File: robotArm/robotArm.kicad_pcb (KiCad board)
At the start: 4 copper layers, 127 x 69.9 mm, 46 parts, among them J1 Barrel_Jack, J2 Conn_01x16_Pin, J3 Conn_01x04, J4 Conn_01x04, J5 Conn_01x04, J6 Conn_01x04, U2 TMC2209_SILENTSTEPSTICK, U4 TMC2209_SILENTSTEPSTICK, U5 TMC2209_SILENTSTEPSTICK, U6 74HC165

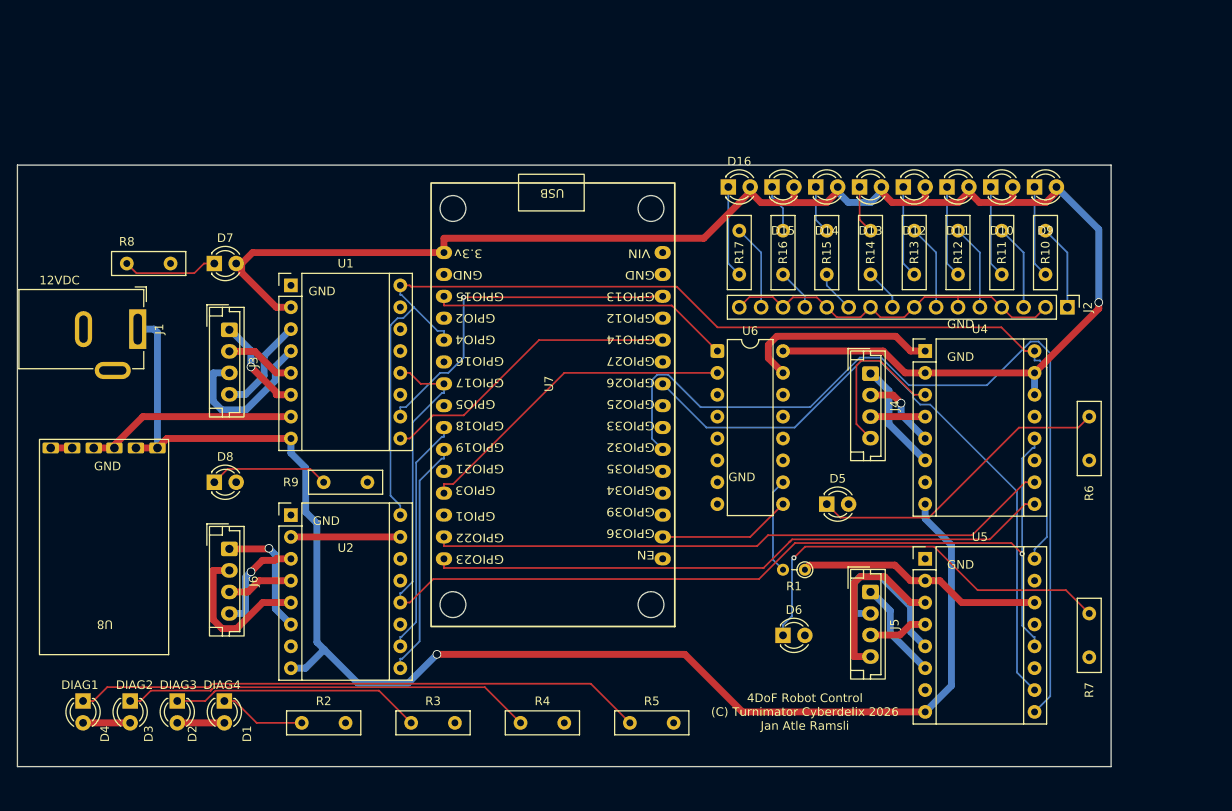
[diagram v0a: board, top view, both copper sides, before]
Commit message: Attempt 2.1
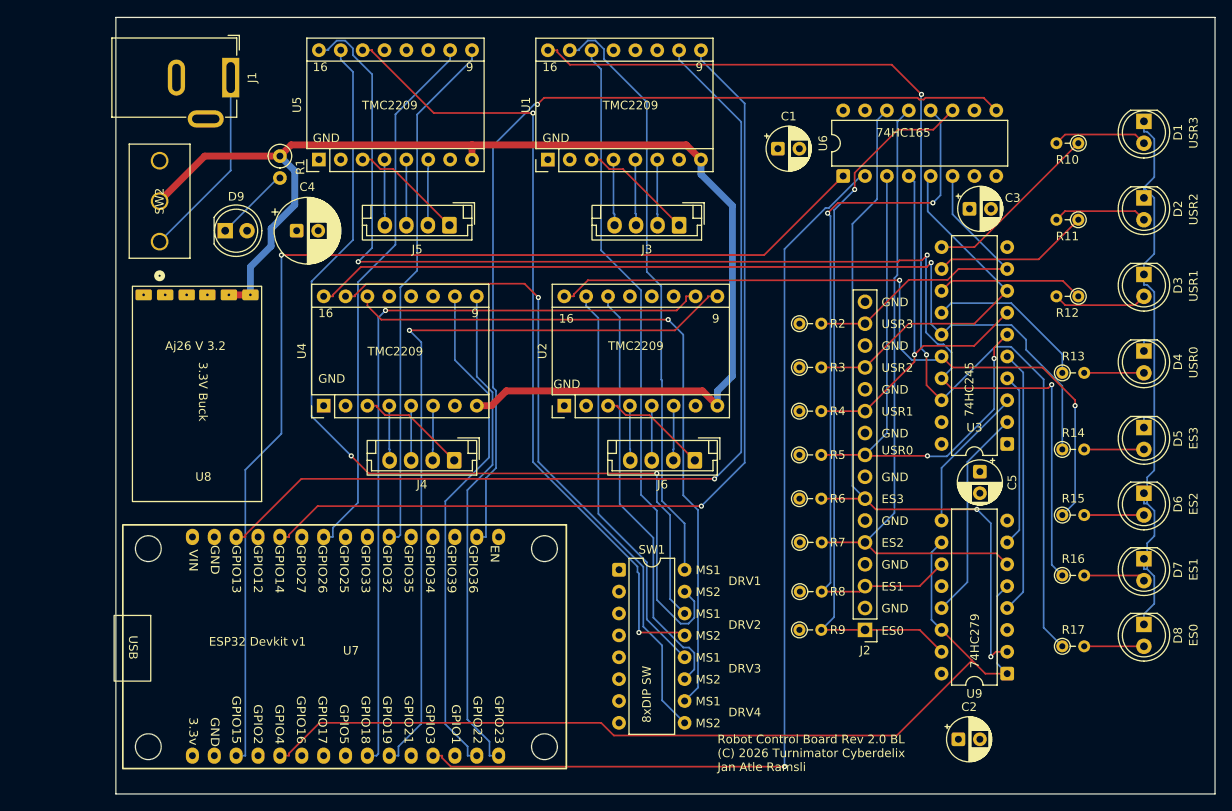
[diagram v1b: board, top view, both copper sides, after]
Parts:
- removed D10: ST1, LED_THT:LED_D3.0mm_FlatTop
- removed D11: ST2, LED_THT:LED_D3.0mm_FlatTop
- removed D12: ST3, LED_THT:LED_D3.0mm_FlatTop
- removed D13: USR0, LED_THT:LED_D3.0mm_FlatTop
- removed D14: USR1, LED_THT:LED_D3.0mm_FlatTop
- removed D15: USR2, LED_THT:LED_D3.0mm_FlatTop
- removed D16: USR3, LED_THT:LED_D3.0mm_FlatTop
- added C1: 47μ, Capacitor_THT:CP_Radial_D5.0mm_P2.50mm, F.Cu at (113.7, 60.3)
- added C2: 47μ, Capacitor_THT:CP_Radial_D5.0mm_P2.50mm, F.Cu at (134.7, 128.9)
- added C3: 47μ, Capacitor_THT:CP_Radial_D5.0mm_P2.50mm, F.Cu at (136.0, 67.3)
- added C4: 100μ, Capacitor_THT:CP_Radial_D7.5mm_P2.50mm, F.Cu at (57.8, 69.8)
- added C5: 47μ, Capacitor_THT:CP_Radial_D5.0mm_P2.50mm, F.Cu at (137.2, 97.8)
- added SW1: SW_DIP_x08, Package_DIP:DIP-16_W7.62mm, F.Cu at (95.3, 109.2)
- added SW2: SW_SPDT, Library:SS-12D10G5_XKB, F.Cu at (41.9, 71.1)
- added U3: 74HC245, Package_DIP:DIP-20_W7.62mm, F.Cu at (140.3, 94.6)
- added U9: 74LS279, Package_DIP:DIP-16_W7.62mm, F.Cu at (140.3, 121.3)
- D1: value DIAG1 -> USR3; footprint LED_THT:LED_D3.0mm_FlatTop -> LED_THT:LED_D5.0mm
- D2: value DIAG2 -> USR2; footprint LED_THT:LED_D3.0mm_FlatTop -> LED_THT:LED_D5.0mm
- D3: value DIAG3 -> USR1; footprint LED_THT:LED_D3.0mm_FlatTop -> LED_THT:LED_D5.0mm
- D4: value DIAG4 -> USR0; footprint LED_THT:LED_D3.0mm_FlatTop -> LED_THT:LED_D5.0mm
- D5: value IX1 -> ES3; footprint LED_THT:LED_D3.0mm_FlatTop -> LED_THT:LED_D5.0mm
- D6: value IX2 -> ES2; footprint LED_THT:LED_D3.0mm_FlatTop -> LED_THT:LED_D5.0mm
- D7: value IX3 -> ES1; footprint LED_THT:LED_D3.0mm_FlatTop -> LED_THT:LED_D5.0mm
- D8: value IX4 -> ES0; footprint LED_THT:LED_D3.0mm_FlatTop -> LED_THT:LED_D5.0mm
- D9: value ST0 -> LED; footprint LED_THT:LED_D3.0mm_FlatTop -> LED_THT:LED_D5.0mm_Clear
- J2: value Conn_01x16_Pin -> ENDSTOP INPUTS
- J3: value Conn_01x04 -> STEPPER1
- J4: value Conn_01x04 -> STEPPER4
- J5: value Conn_01x04 -> STEPPER2
- J6: value Conn_01x04 -> STEPPER3
- R1: value R -> 470 Ω; footprint Resistor_THT:R_Axial_DIN0204_L3.6mm_D1.6mm_P2.54mm_Vertical -> Resistor_THT:R_Axial_DIN0207_L6.3mm_D2.5mm_P2.54mm_Vertical
- R10, R11, R12, R13, R14, R15, R16, R17: value 330 -> 330Ω; footprint Resistor_THT:R_Box_L8.4mm_W2.5mm_P5.08mm -> Resistor_THT:R_Axial_DIN0204_L3.6mm_D1.6mm_P2.54mm_Vertical
- R2, R3, R4, R5, R6, R7, R8, R9: value 330 -> 10kΩ; footprint Resistor_THT:R_Box_L8.4mm_W2.5mm_P5.08mm -> Resistor_THT:R_Axial_DIN0204_L3.6mm_D1.6mm_P2.54mm_Vertical
- U4: value TMC2209_SILENTSTEPSTICK -> TMC2209_MODULE
- U5: value TMC2209_SILENTSTEPSTICK -> TMC2209 Module
- moved D4 129.7 mm to (156.2, 83.8)
- moved D3 127.7 mm to (156.2, 74.9)
- moved D2 126.5 mm to (156.2, 66.0)
- moved D1 126.2 mm to (156.2, 57.1)
- moved D7 113.3 mm to (156.2, 108.0), turned to -90 degrees
- moved D8 109.2 mm to (156.2, 115.6), turned to -90 degrees
- moved D9 94.1 mm to (49.5, 69.8)
- moved R8 86.9 mm to (116.3, 111.8)
- moved U5 84.3 mm to (60.4, 61.6), turned to 90 degrees
- moved R1 77.6 mm to (55.9, 61.2), turned to -90 degrees
- moved R2 74.1 mm to (116.2, 80.6)
- moved U4 70.1 mm to (61.0, 90.2), turned to 90 degrees
- moved J5 64.8 mm to (75.6, 69.2), turned to 180 degrees
- moved R3 61.1 mm to (116.2, 85.7)
- moved R9 57.8 mm to (116.2, 116.2)
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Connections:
- D1 pad 2: +3.3V -> Net-(D1-A)
- D2 pad 1: Net-(D2-K) -> Net-(D1-K)
- D2 pad 2: +3.3V -> Net-(D2-A)
- D3 pad 1: Net-(D3-K) -> Net-(D1-K)
- D3 pad 2: +3.3V -> Net-(D3-A)
- D4 pad 1: Net-(D4-K) -> Net-(D1-K)
- D4 pad 2: +3.3V -> Net-(D4-A)
- D5 pad 1: Net-(D5-K) -> Net-(D1-K)
- D5 pad 2: +3.3V -> Net-(D5-A)
- D6 pad 1: Net-(D6-K) -> Net-(D1-K)
- D6 pad 2: +3.3V -> Net-(D6-A)
- D7 pad 1: Net-(D7-K) -> Net-(D1-K)
- D7 pad 2: +3.3V -> Net-(D7-A)
- D8 pad 1: Net-(D8-K) -> Net-(D1-K)
- D8 pad 2: +3.3V -> Net-(D8-A)
- D9 pad 2: +3.3V -> GND
- J1 pad 1: +12V -> Net-(J1-Pad1)
- J2 pad 1: ES0 -> /Endstop Section/ES0
- J2 pad 10: Net-(J2-Pin_10) -> GND
- J2 pad 11: USR1 -> /Endstop Section/USR1
- J2 pad 12: Net-(J2-Pin_10) -> GND
- J2 pad 13: USR2 -> /Endstop Section/USR2
- J2 pad 14: Net-(J2-Pin_10) -> GND
- J2 pad 15: USR3 -> /Endstop Section/USR3
- J2 pad 16: Net-(J2-Pin_10) -> GND
- J2 pad 2: Net-(J2-Pin_10) -> GND
- J2 pad 3: ES1 -> /Endstop Section/ES1
- J2 pad 4: Net-(J2-Pin_10) -> GND
- J2 pad 5: ES2 -> /Endstop Section/ES2
- J2 pad 6: Net-(J2-Pin_10) -> GND
- J2 pad 7: ES3 -> /Endstop Section/ES3
- J2 pad 8: Net-(J2-Pin_10) -> GND
- J2 pad 9: USR0 -> /Endstop Section/USR0
- J3 pad 1: /M1-2B -> /B2-DRV1
- J3 pad 2: /M1-2A -> /A2-DRV1
- J3 pad 3: /M1-1A -> /A1-DRV1
- J3 pad 4: /M1-1B -> /B1-DRV1
- J4 pad 1: /M4-1B -> /B2-DRV4
- J4 pad 2: /M4-2A -> /A2-DRV4
- J4 pad 3: /M4-1A -> /A1-DRV4
- J4 pad 4: Net-(J4-2B) -> /B1-DRV4
- J5 pad 1: /M2-2B -> /B2-DRV2
- J5 pad 2: /M2-2A -> /A2-DRV2
- J5 pad 3: /M2-1A -> /A1-DRV2
- J5 pad 4: /M2-1B -> /B1-DRV2
- J6 pad 1: /M3-2B -> /B2-DRV3
- J6 pad 2: /M3-2A -> /A2-DRV3
- J6 pad 3: /M3-1A -> /A1-DRV3
- J6 pad 4: /M3-1B -> /B1-DRV3
- R1 pad 1: +3.3V -> +12V
- R1 pad 2: Net-(U6-DS) -> Net-(D9-K)
- R10 pad 1: Net-(D9-K) -> Net-(U3-B7)
- R10 pad 2: ES0 -> Net-(D1-A)
- R11 pad 2: ES1 -> Net-(D2-A)
- R12 pad 2: ES2 -> Net-(D3-A)
- R13 pad 2: ES3 -> Net-(D4-A)
- R14 pad 1: Net-(D13-K) -> /EN_DRV4
- R14 pad 2: USR0 -> Net-(D5-A)
- R15 pad 1: Net-(D14-K) -> /EN_DRV3
- R15 pad 2: USR1 -> Net-(D6-A)
- R16 pad 1: Net-(D15-K) -> /EN_DRV2
- R16 pad 2: USR2 -> Net-(D7-A)
- R17 pad 1: Net-(D16-K) -> /EN_DRV1
- R17 pad 2: USR3 -> Net-(D8-A)
- R2 pad 1: Net-(D1-K) -> +3.3V
- R2 pad 2: DIAG1 -> /Endstop Section/USR3
- R3 pad 1: Net-(D2-K) -> +3.3V
- R3 pad 2: DIAG2 -> /Endstop Section/USR2
- R4 pad 1: Net-(D3-K) -> +3.3V
- R4 pad 2: DIAG3 -> /Endstop Section/USR1
- R5 pad 1: Net-(D4-K) -> +3.3V
- R5 pad 2: DIAG4 -> /Endstop Section/USR0
- R6 pad 1: Net-(D5-K) -> +3.3V
- R6 pad 2: IX1 -> /Endstop Section/ES3
- R7 pad 1: Net-(D6-K) -> +3.3V
- R7 pad 2: IX2 -> /Endstop Section/ES2
- R8 pad 1: Net-(D7-K) -> +3.3V
- R8 pad 2: IX3 -> /Endstop Section/ES1
- R9 pad 1: Net-(D8-K) -> +3.3V
- R9 pad 2: IX4 -> /Endstop Section/ES0
- U1 pad 11: unconnected-(U1-PDN-Pad11) -> GND
- U1 pad 12: UART2_TX -> unconnected-(U1-TX-Pad12)
- U1 pad 14: unconnected-(U1-MS2-Pad14) -> MS2-DRV1
- U1 pad 15: unconnected-(U1-MS1-Pad15) -> MS1-DRV1
- U1 pad 16: EN_DRV -> /EN_DRV1
- U1 pad 3: /M1-1B -> /B2-DRV1
- U1 pad 4: /M1-1A -> /B1-DRV1
- U1 pad 5: /M1-2A -> /A1-DRV1
- U1 pad 6: /M1-2B -> /A2-DRV1
- U2 pad 11: unconnected-(U2-PDN-Pad11) -> GND
- U2 pad 12: UART2_TX -> unconnected-(U2-TX-Pad12)
- U2 pad 14: unconnected-(U2-MS2-Pad14) -> MS2-DRV3
- U2 pad 15: +3.3V -> MS1-DRV3
- U2 pad 16: EN_DRV -> /EN_DRV3
- U2 pad 3: /M3-1B -> /B2-DRV3
- U2 pad 4: /M3-1A -> /B1-DRV3
- U2 pad 5: /M3-2A -> /A1-DRV3
- U2 pad 6: /M3-2B -> /A2-DRV3
- U4 pad 11: unconnected-(U4-PDN-Pad11) -> GND
- U4 pad 12: UART2_TX -> unconnected-(U4-TX-Pad12)
- U4 pad 14: +3.3V -> MS1-DRV4
- U4 pad 15: +3.3V -> MS2-DRV4
- U4 pad 16: EN_DRV -> /EN_DRV4
- U4 pad 3: Net-(J4-2B) -> /B2-DRV4
- U4 pad 4: /M4-1A -> /B1-DRV4
- U4 pad 5: /M4-2A -> /A1-DRV4
- U4 pad 6: /M4-1B -> /A2-DRV4
- U5 pad 11: unconnected-(U5-PDN-Pad11) -> GND
- U5 pad 12: UART2_TX -> unconnected-(U5-TX-Pad12)
- U5 pad 14: +3.3V -> MS2-DRV2
- U5 pad 15: unconnected-(U5-MS1-Pad15) -> MS1-DRV2
- U5 pad 16: EN_DRV -> /EN_DRV2
- U5 pad 3: /M2-1B -> /B2-DRV2
- U5 pad 4: /M2-1A -> /B1-DRV2
- U5 pad 5: /M2-2A -> /A1-DRV2
- U5 pad 6: /M2-2B -> /A2-DRV2
- U6 pad 10: Net-(U6-DS) -> GND
- U6 pad 11: D0 -> /Endstop Section/ES0
- U6 pad 12: D1 -> /Endstop Section/ES1
- U6 pad 13: D2 -> /Endstop Section/ES2
- U6 pad 14: D3 -> /Endstop Section/ES3
- U6 pad 3: D4 -> /Endstop Section/USR0
- U6 pad 4: D5 -> /Endstop Section/USR1
- U6 pad 5: D6 -> /Endstop Section/USR2
- U6 pad 6: D7 -> /Endstop Section/USR3
- U7 pad 20: EN_DRV -> /RESET_DRV
- U7 pad 22: UART2_TX -> unconnected-(U7-GPIO17-Pad22)
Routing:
- net +3.3V: track 236.0 -> 0.00 mm, vias 1 -> 0
- net /EN_DRV2: track 0.00 -> 150.3 mm, vias 0 -> 3
- net EN_DRV: track 137.6 -> 0.00 mm
- net UART2_TX: track 134.4 -> 0.00 mm, vias 1 -> 0
- net /EN_DRV1: track 0.00 -> 130.1 mm, vias 0 -> 2
- net /RESET_DRV: track 0.00 -> 118.3 mm
- net /EN_DRV4: track 0.00 -> 106.6 mm, vias 0 -> 1
- net MS1-DRV2: track 0.00 -> 105.5 mm, vias 0 -> 2
- net LOAD: track 35.0 -> 130.0 mm, vias 0 -> 1
- net MS2-DRV2: track 0.00 -> 93.7 mm, vias 0 -> 2
- net DATA: track 15.5 -> 108.7 mm, vias 0 -> 1
- net /Endstop Section/ES3: track 0.00 -> 85.9 mm, vias 0 -> 2
- net /EN_DRV3: track 0.00 -> 84.9 mm, vias 0 -> 2
- net /Endstop Section/ES0: track 0.00 -> 84.1 mm, vias 0 -> 1
- net /Endstop Section/ES1: track 0.00 -> 84.0 mm, vias 0 -> 2
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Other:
- board size 127 x 69.9 mm -> 127.6 x 90.2 mm
- board text added: "16"
- board text added: "74HC165"
- board text added: "74HC245"
- board text added: "74HC279"
- board text added: "8xDIP SW"
- board text added: "9"
- board text added: "Aj26 V 3.2"
- board text added: "DRV1"
- board text added: "DRV2"
- board text added: "DRV3"
- board text added: "DRV4"
- board text added: "ES0"
- board text added: "ES1"
- board text added: "ES2"
- board text added: "ES3"
- board text added: "ESP32 Devkit v1"
- board text added: "MS1"
- board text added: "MS2"
- board text added: "Robot Control Board Rev 2.0 BL (C) 2026 Turnimator Cyberdelix Jan Atle Ramsli"
- board text added: "TMC2209"
- board text added: "USR0"
- board text added: "USR1"
- board text added: "USR2"
- board text added: "USR3"
- board text removed: "12VDC"
- board text removed: "4DoF Robot Control (C) Turnimator Cyberdelix 2026 Jan Atle Ramsli"
- board text removed: "DIAG1"
- board text removed: "DIAG2"
- board text removed: "DIAG3"
- board text removed: "DIAG4"
